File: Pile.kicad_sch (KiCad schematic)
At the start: 17 parts, among them J41 Conn_PH_01x16

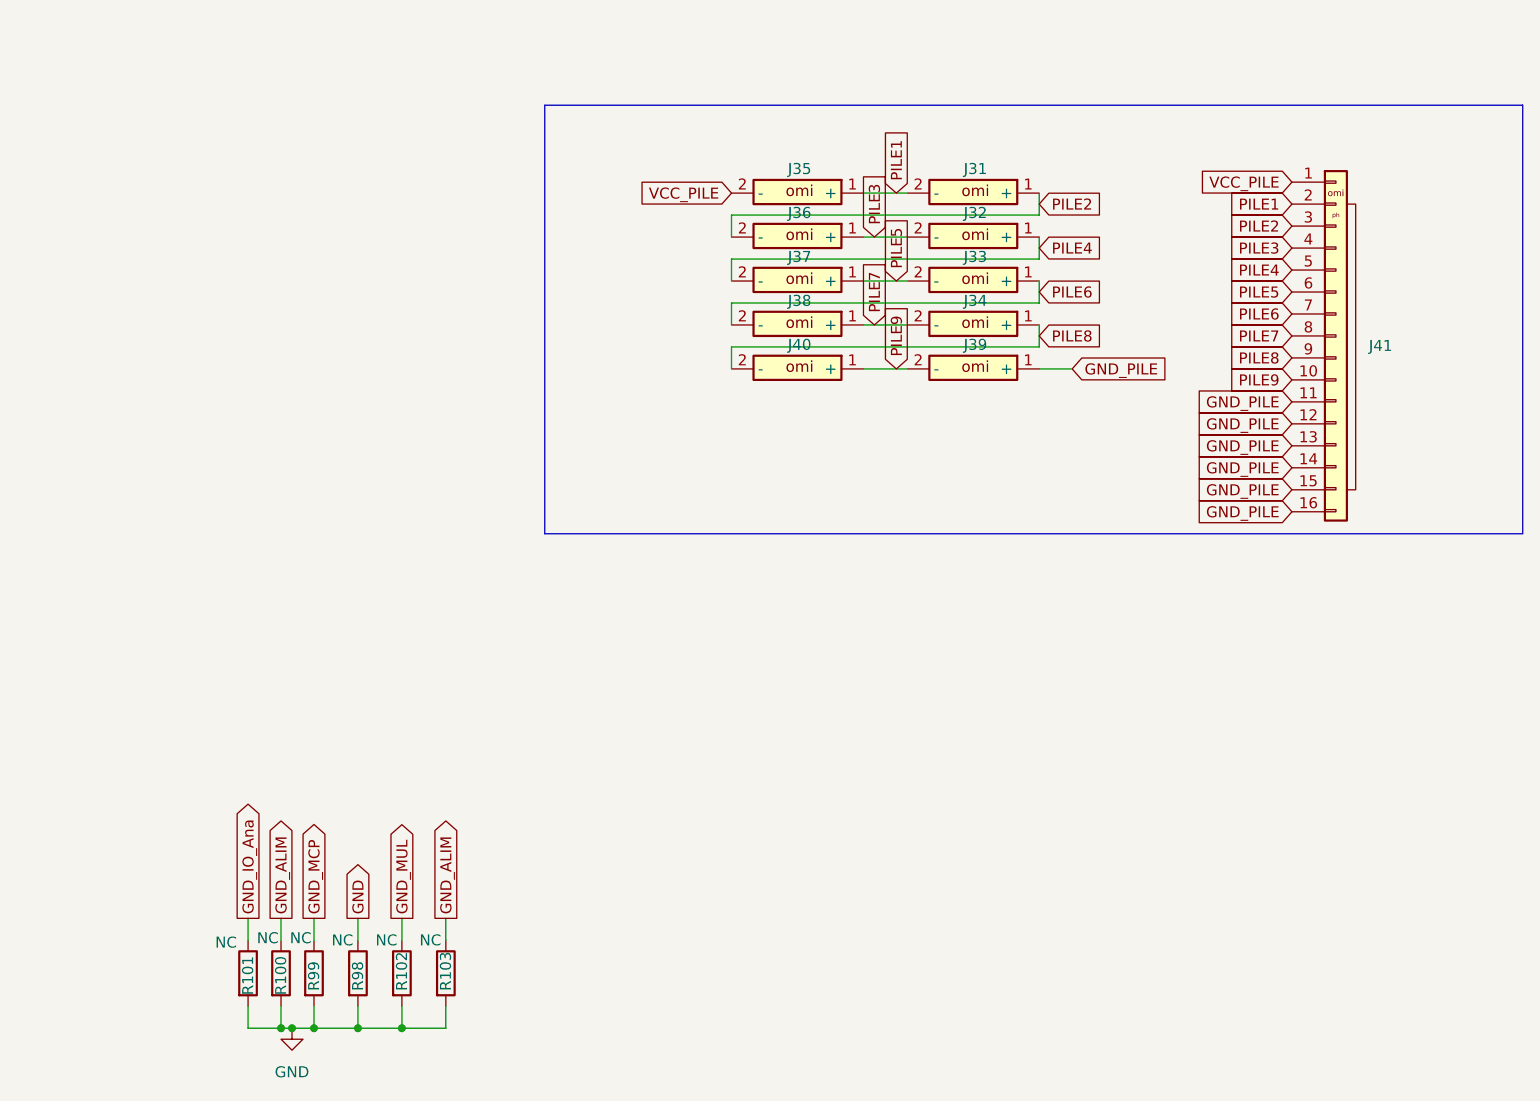
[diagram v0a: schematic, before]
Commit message: 26/06/2025  11:50 Signed-off-by: TEST-BANC <TEST-BANC@DOMOMICRON.LOCAL>
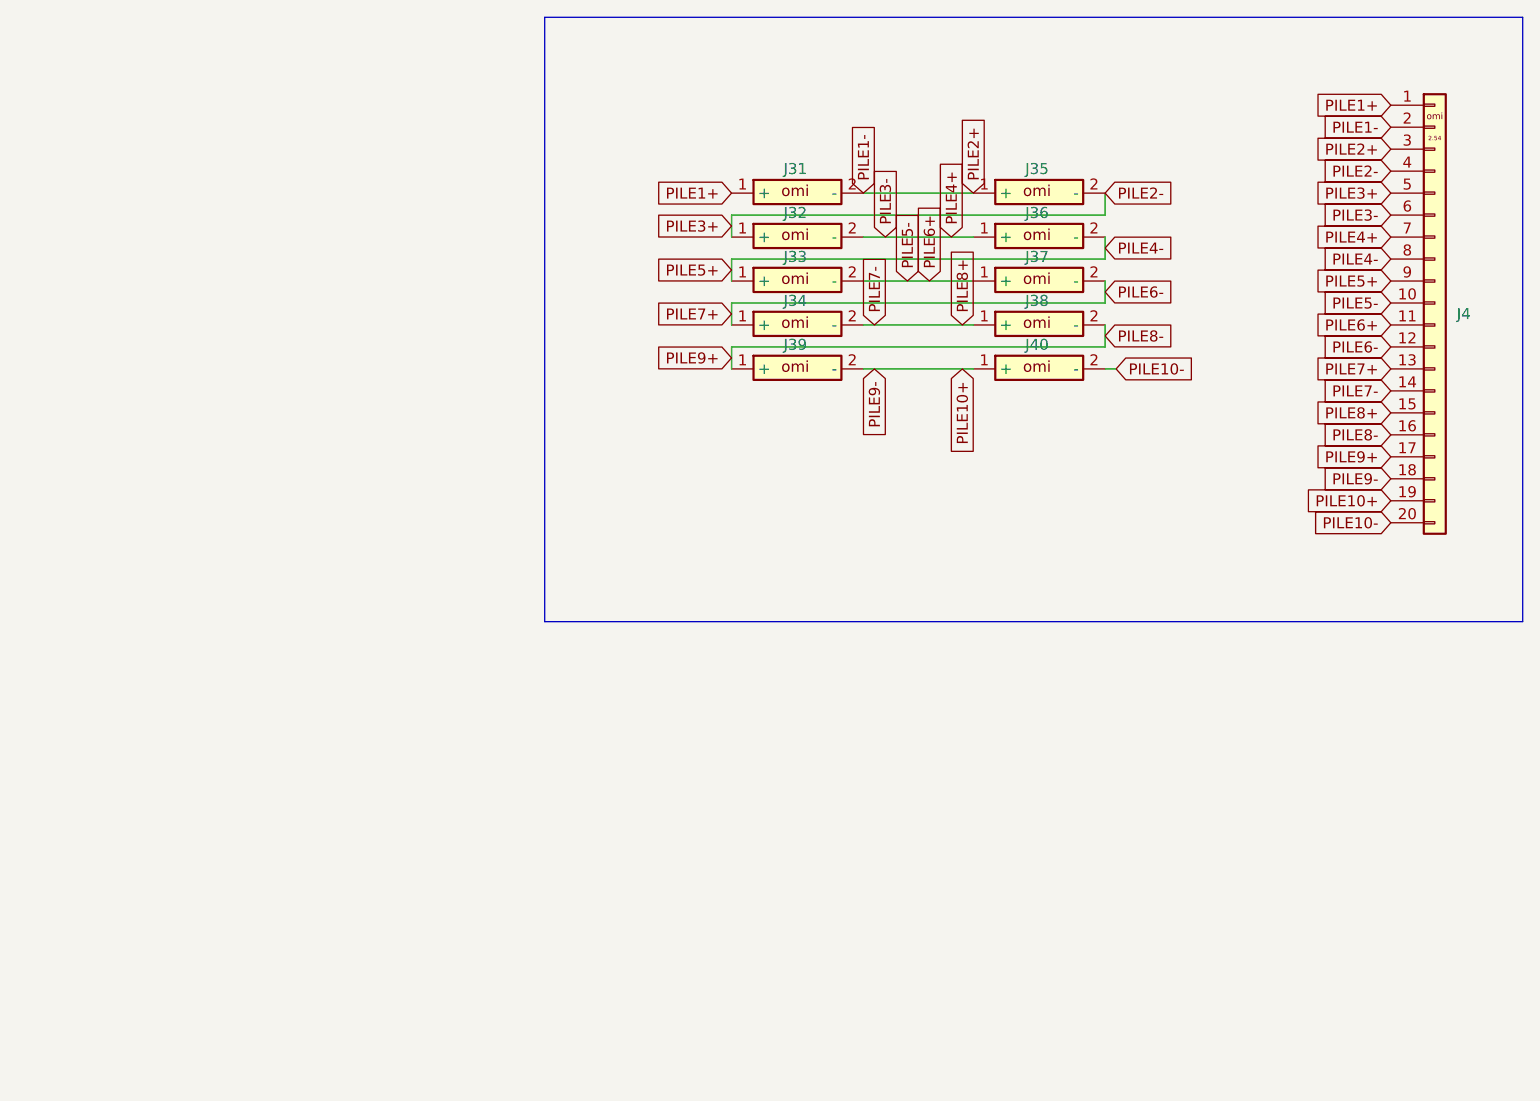
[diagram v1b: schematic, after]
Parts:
- removed J41: Conn_PH_01x16, symbol Omiconnecteur:Conn_PH_01x16_P2.00mm_trad_vertical
- removed R100, R101, R102, R103, R98, R99: NC, symbol Device:R
- added J4: Conn_01x32_P2.54mm_pinheader_vertical, Omiconnecteur:PinHeader_1x32_P2.54mm_V_omi, symbol Omiconnecteur:Conn_01x20_P2.54mm_pinheader_vertical
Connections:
- net VCC_PILE is gone; now on net PILE2-: J35.2 (-)
- net GND_PILE renamed PILE8-
- net PILE8-: now also J38.2 (-), J4.16 (Pin_16), J4.17 (Pin_17)
- net PILE1 renamed PILE1-
- net PILE1-: now also J4.2 (Pin_2), J4.3 (Pin_3)
- net PILE2 renamed PILE1+
- net PILE1+: now also J4.1 (Pin_1); no longer J36.2 (-)
- net PILE3 renamed PILE3-
- net PILE3-: now also J4.6 (Pin_6), J4.7 (Pin_7)
- net PILE4 renamed PILE2-
- net PILE2-: now also J4.4 (Pin_4), J4.5 (Pin_5); no longer J37.2 (-)
- net PILE5 renamed PILE5-
- net PILE5-: now also J4.10 (Pin_10), J4.11 (Pin_11)
- net PILE6 renamed PILE4-
- net PILE4-: now also J36.2 (-), J4.8 (Pin_8), J4.9 (Pin_9); no longer J38.2 (-)
- net PILE7 renamed PILE7-
- net PILE7-: now also J4.14 (Pin_14), J4.15 (Pin_15)
- net PILE8 renamed PILE10-
- net PILE10-: now also J4.20 (Pin_20); no longer J34.1 (+)
- net PILE9 renamed PILE10+
- net PILE10+: now also J4.18 (Pin_18), J4.19 (Pin_19)
- new net PILE6-: J34.1 (+), J37.2 (-), J4.12 (Pin_12), J4.13 (Pin_13)
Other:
- moved on the sheet: J31, J32, J33, J34, J35, J36, J37, J38, J39, J40

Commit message: 26/06/2025  14:23 Signed-off-by: TEST-BANC <TEST-BANC@DOMOMICRON.LOCAL>
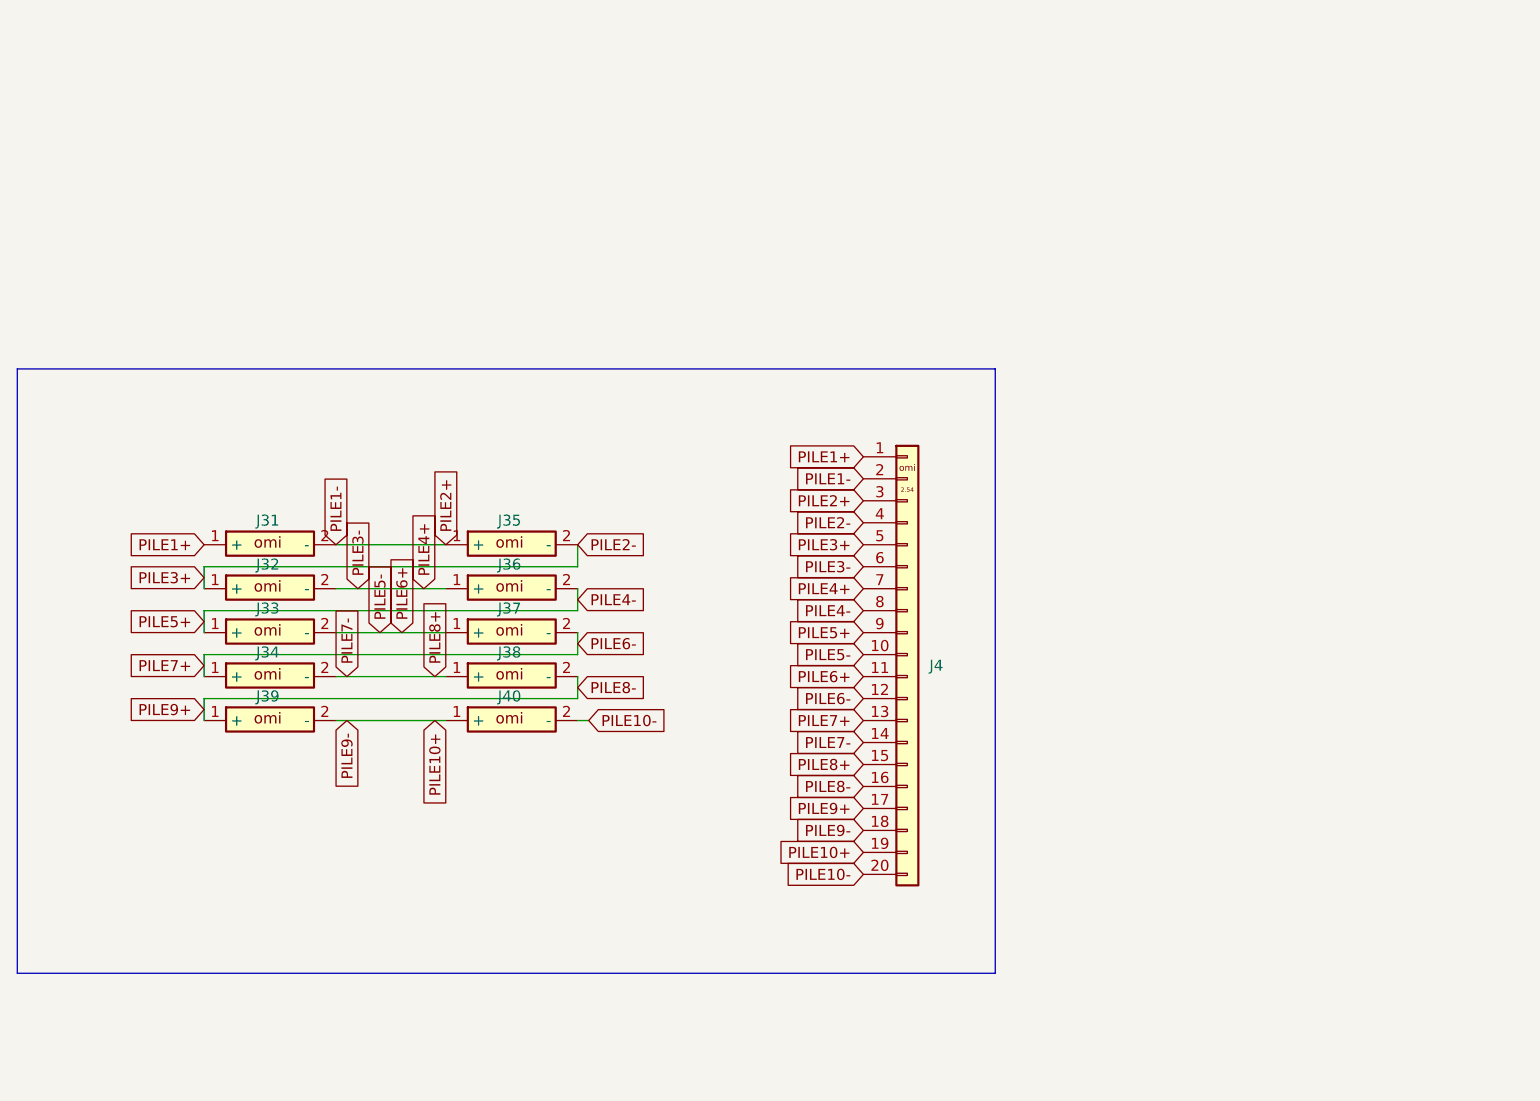
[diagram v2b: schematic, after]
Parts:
- J31, J32, J33, J34, J35, J36, J37, J38, J39, J40: footprint (none) -> Omialimentation:BAT_1075; Distributeur1 (none) -> M:534-1075; Distributeur2 (none) -> DK:36-1075-ND 1075; Fabreference (none) -> 1075; Farbiquant (none) -> Keystone Electronics; Omicron (none) -> ACO005137
- J4: value Conn_01x32_P2.54mm_pinheader_vertical -> Conn_01x20_P2.54mm_pinheader_vertical; footprint Omiconnecteur:PinHeader_1x32_P2.54mm_V_omi -> Omiconnecteur:PinHeader_1x20_P2.54mm_V_omi
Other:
- moved on the sheet: J31, J32, J33, J34, J35, J36, J37, J38, J39, J4, J40
